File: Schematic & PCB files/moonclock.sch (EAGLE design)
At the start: 27 parts, among them U1 TCA9548APWR, U2 ESP32-S2-WROVER-I, U3 AMS1117-3.3, X2 BM04B-SRSS-TB

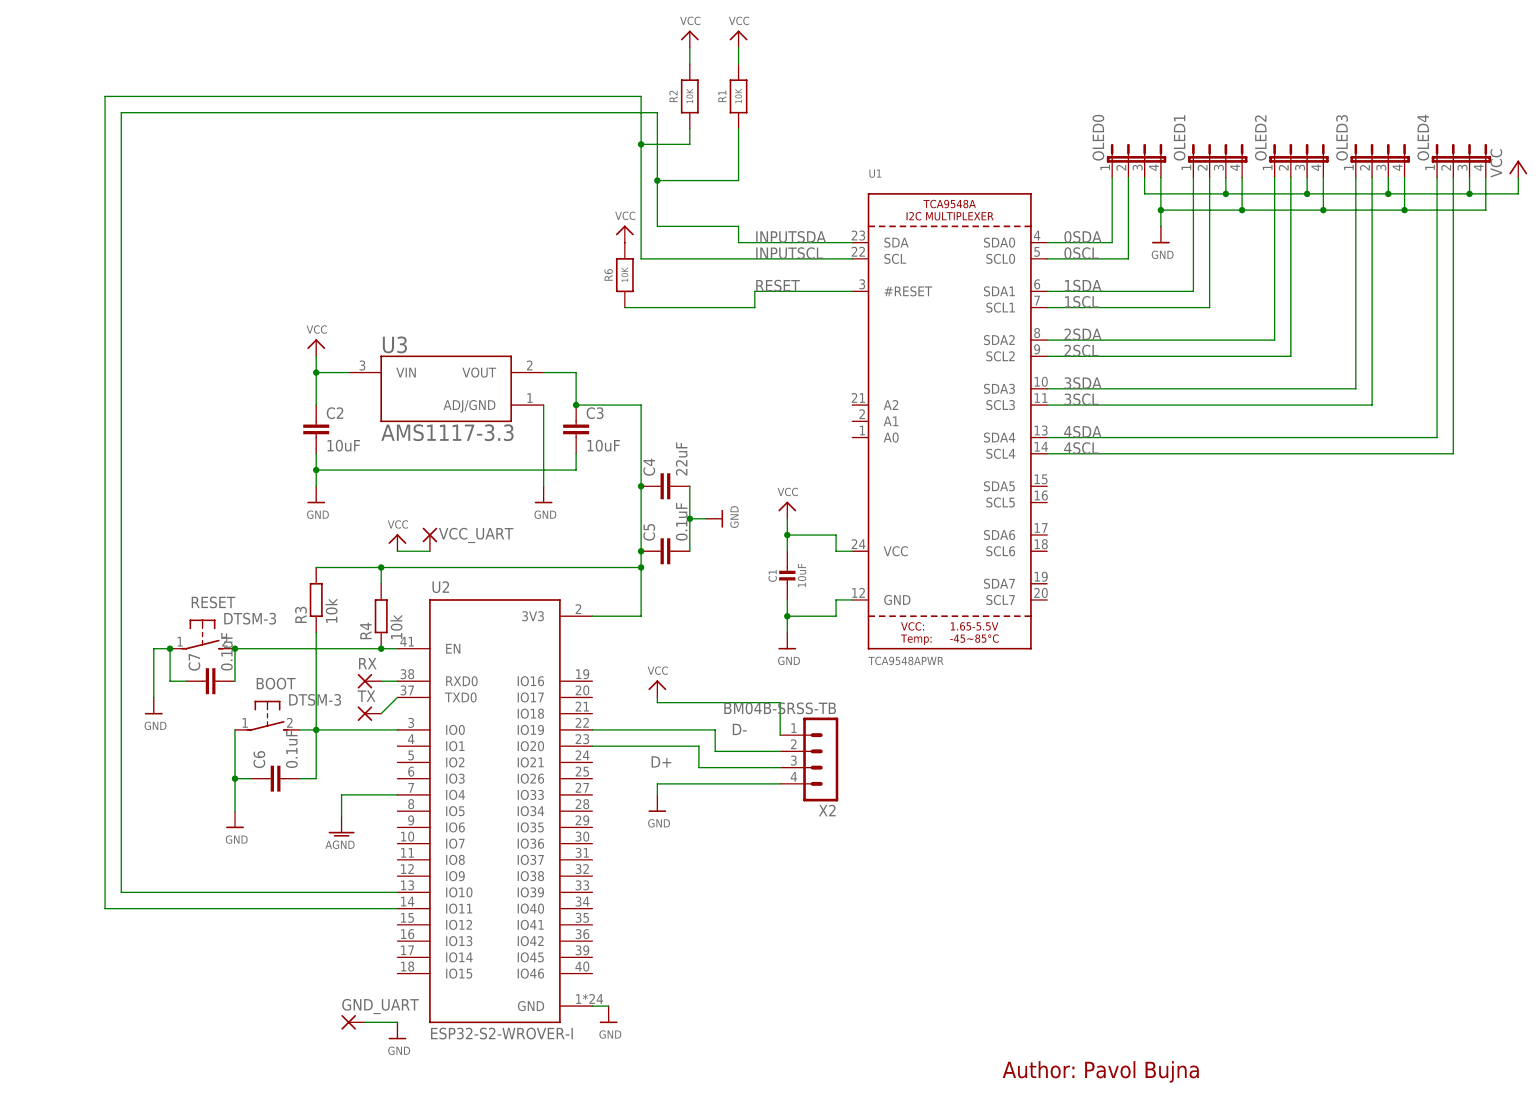
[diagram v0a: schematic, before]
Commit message: PCB
feat: MoonClock add schematics and pcb files
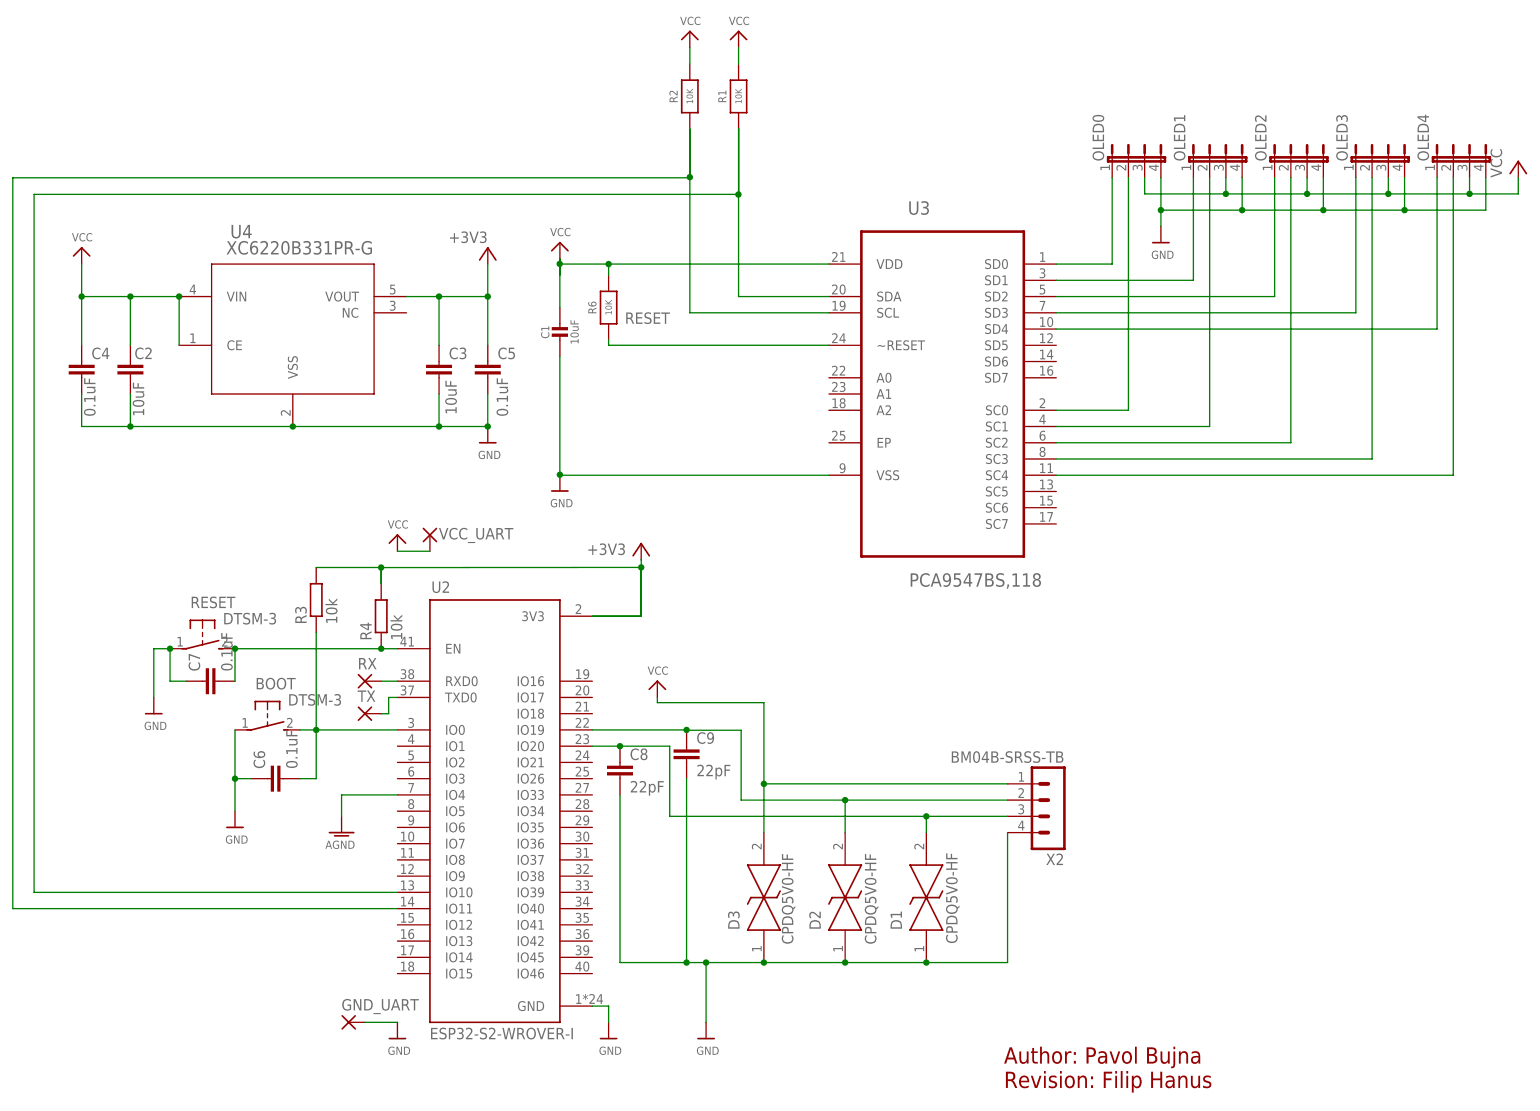
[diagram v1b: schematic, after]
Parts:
- removed U1: TCA9548APWR, microbuilder:TCA9548A
- added C8, C9: 22pF, rcl:C-EUC0805
- added D1, D2, D3: CPDQ5V0-HF, CPDQ5V0-HF:CPDQ5V0-HF
- added U4: XC6220B331PR-G, tribonix:XC6220B331PR-G
- C4: value 22uF -> 0.1uF
- U3: value AMS1117-3.3 -> PCA9547BS,118; device AMS1117-3.3:AMS1117-3.3 -> PCA9547BS_118:PCA9547BS,118
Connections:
- removed net 0SCL: OLED0.2, U1.SCL0
- removed net 0SDA: OLED0.1, U1.SDA0
- removed net 1SCL: OLED1.2, U1.SCL1
- removed net 1SDA: OLED1.1, U1.SDA1
- removed net 2SCL: OLED2.2, U1.SCL2
- removed net 2SDA: OLED2.1, U1.SDA2
- removed net 3SCL: OLED3.2, U1.SCL3
- removed net 3SDA: OLED3.1, U1.SDA3
- removed net 4SCL: OLED4.2, U1.SCL4
- removed net 4SDA: OLED4.1, U1.SDA4
- removed net INPUTSCL: R2.1, U1.SCL, U2.IO11
- removed net INPUTSDA: R1.1, U1.SDA, U2.IO10
- new net +3V3: C3.1, C5.1, R3.2, R4.2, U4.VOUT
- new net N$1: U2.3V3
- new net N$11: OLED3.1, U3.SD3
- new net N$12: OLED4.1, U3.SD4
- new net N$13: OLED0.2, U3.SC0
- new net N$14: OLED1.2, U3.SC1
- new net N$15: OLED2.2, U3.SC2
- new net N$16: OLED3.2, U3.SC3
- new net N$17: OLED4.2, U3.SC4
- new net N$2: R1.1, U2.IO10, U3.SDA
- new net N$3: R2.1, U2.IO11, U3.SCL
- new net N$4: OLED0.1, U3.SD0
- new net N$9: OLED2.1, U3.SD2
- net D+: now also C8.1, D1.A
- net D-: now also C9.1, D2.A
- net GND: now also C8.2, C9.2, D1.K, D2.K, D3.K, U3.VSS, U4.VSS; no longer U1.GND, U3.ADJ/GND
- net N$7: now also OLED1.1, U3.SD1; no longer C3.1, C4.1, C5.1, R3.2, R4.2, U2.3V3, U3.VOUT
- net RESET: now also U3.~RESET; no longer U1.#RESET
- net VCC: now also C4.1, D3.A, U3.VDD, U4.CE, U4.VIN; no longer U1.VCC, U3.VIN
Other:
- note added: "Author: Pavol Bujna Revision: Filip Hanus"
- note removed: "Author: Pavol Bujna"
- moved on the sheet: C1, C2, C3, C4, C5, R6, X2
